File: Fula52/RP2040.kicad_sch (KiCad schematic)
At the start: 25 parts, among them SW1 BOOT, SW2 RESET, U3 W25Q128JVS, U4 RP2040, Y1 12MHz

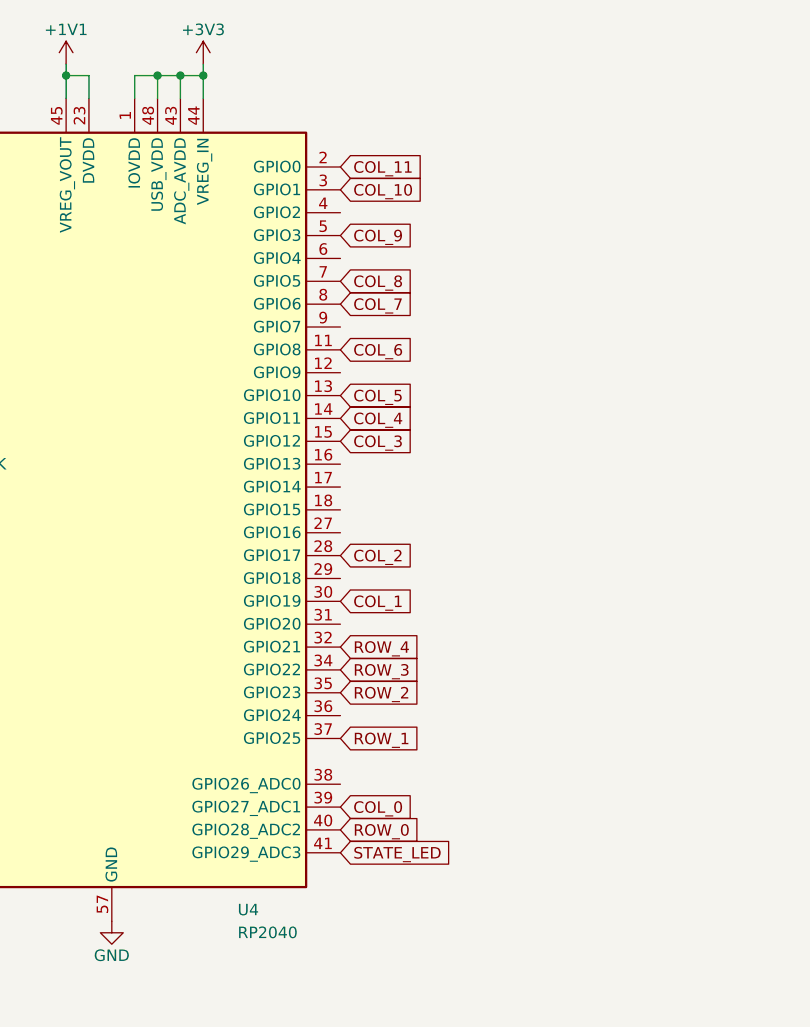
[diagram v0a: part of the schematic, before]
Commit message: full routed
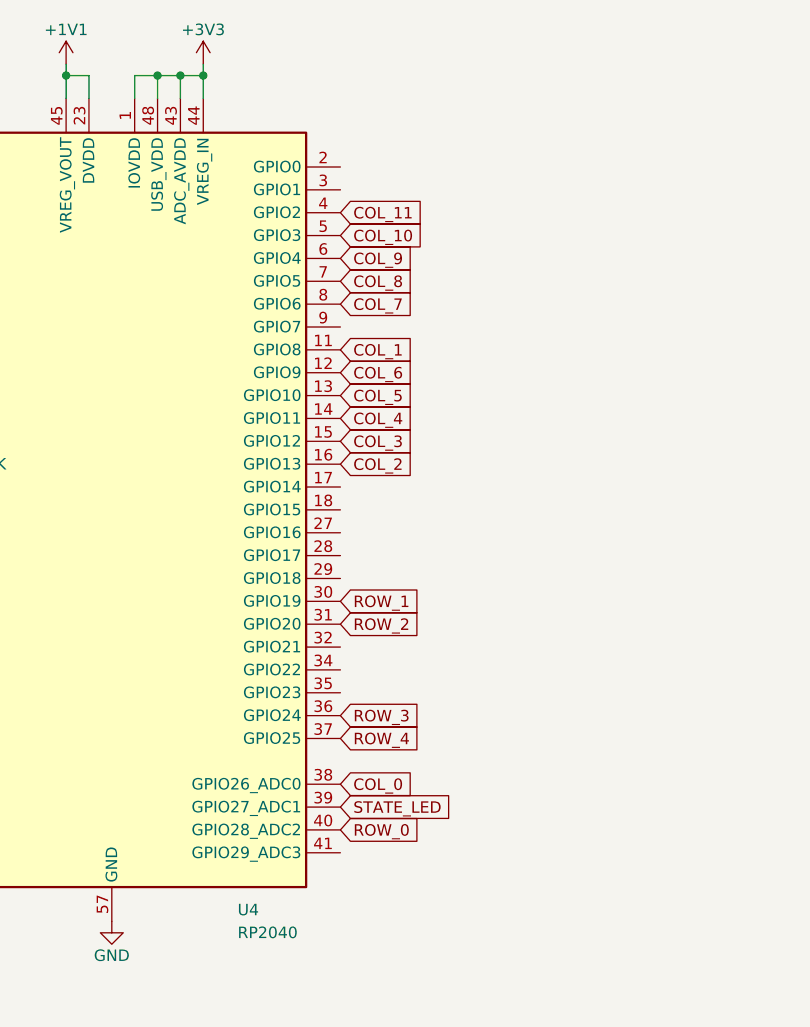
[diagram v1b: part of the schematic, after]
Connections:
- net COL_0: now also U4.38 (GPIO26_ADC0); no longer U4.39 (GPIO27_ADC1)
- net COL_1: now also U4.11 (GPIO8); no longer U4.30 (GPIO19)
- net COL_10: now also U4.5 (GPIO3); no longer U4.3 (GPIO1)
- net COL_11: now also U4.4 (GPIO2); no longer U4.2 (GPIO0)
- net COL_2: now also U4.16 (GPIO13); no longer U4.28 (GPIO17)
- net COL_6: now also U4.12 (GPIO9); no longer U4.11 (GPIO8)
- net COL_9: now also U4.6 (GPIO4); no longer U4.5 (GPIO3)
- net ROW_1: now also U4.30 (GPIO19); no longer U4.37 (GPIO25)
- net ROW_2: now also U4.31 (GPIO20); no longer U4.35 (GPIO23)
- net ROW_3: now also U4.36 (GPIO24); no longer U4.34 (GPIO22)
- net ROW_4: now also U4.37 (GPIO25); no longer U4.32 (GPIO21)
- net STATE_LED: now also U4.39 (GPIO27_ADC1); no longer U4.41 (GPIO29_ADC3)
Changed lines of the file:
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@@
     (effects (font (size 1.27 1.27)) (justify right bottom))
   )
-  (global_label "COL_2" (shape input) (at 116.84 83.82 0) (fields_autoplaced)
+  (global_label "COL_2" (shape input) (at 116.84 73.66 0) (fields_autoplaced)
     (effects (font (size 1.27 1.27)) (justify left))
-    (property "Intersheet References" "${INTERSHEET_REFS}" (id 0) (at 125.0588 83.7406 0)
+    (property "Intersheet References" "${INTERSHEET_REFS}" (id 0) (at 125.0588 73.5806 0)
       (effects (font (size 1.27 1.27)) (justify left) hide)
     )
   )
-  (global_label "ROW_1" (shape input) (at 116.84 104.14 0) (fields_autoplaced)
+  (global_label "ROW_1" (shape input) (at 116.84 88.9 0) (fields_autoplaced)
     (effects (font (size 1.27 1.27)) (justify left))
-    (property "Intersheet References" "${INTERSHEET_REFS}" (id 0) (at 125.4821 104.0606 0)
+    (property "Intersheet References" "${INTERSHEET_REFS}" (id 0) (at 125.4821 88.8206 0)
       (effects (font (size 1.27 1.27)) (justify left) hide)
     )
@@
     )
   )
-  (global_label "COL_10" (shape input) (at 116.84 43.18 0) (fields_autoplaced)
+  (global_label "COL_10" (shape input) (at 116.84 48.26 0) (fields_autoplaced)
     (effects (font (size 1.27 1.27)) (justify left))
-    (property "Intersheet References" "${INTERSHEET_REFS}" (id 0) (at 126.2683 43.1006 0)
+    (property "Intersheet References" "${INTERSHEET_REFS}" (id 0) (at 126.2683 48.1806 0)
       (effects (font (size 1.27 1.27)) (justify left) hide)
     )
@@
     )
   )
-  (global_label "COL_0" (shape input) (at 116.84 111.76 0) (fields_autoplaced)
+  (global_label "COL_0" (shape input) (at 116.84 109.22 0) (fields_autoplaced)
     (effects (font (size 1.27 1.27)) (justify left))
-    (property "Intersheet References" "${INTERSHEET_REFS}" (id 0) (at 125.0588 111.6806 0)
+    (property "Intersheet References" "${INTERSHEET_REFS}" (id 0) (at 125.0588 109.1406 0)
       (effects (font (size 1.27 1.27)) (justify left) hide)
     )
   )
-  (global_label "COL_9" (shape input) (at 116.84 48.26 0) (fields_autoplaced)
+  (global_label "COL_9" (shape input) (at 116.84 50.8 0) (fields_autoplaced)
     (effects (font (size 1.27 1.27)) (justify left))
-    (property "Intersheet References" "${INTERSHEET_REFS}" (id 0) (at 125.0588 48.1806 0)
+    (property "Intersheet References" "${INTERSHEET_REFS}" (id 0) (at 125.0588 50.7206 0)
       (effects (font (size 1.27 1.27)) (justify left) hide)
     )
   )
-  (global_label "ROW_4" (shape input) (at 116.84 93.98 0) (fields_autoplaced)
+  (global_label "ROW_4" (shape input) (at 116.84 104.14 0) (fields_autoplaced)
     (effects (font (size 1.27 1.27)) (justify left))
-    (property "Intersheet References" "${INTERSHEET_REFS}" (id 0) (at 125.4821 93.9006 0)
+    (property "Intersheet References" "${INTERSHEET_REFS}" (id 0) (at 125.4821 104.0606 0)
       (effects (font (size 1.27 1.27)) (justify left) hide)
     )
   )
-  (global_label "COL_11" (shape input) (at 116.84 40.64 0) (fields_autoplaced)
+  (global_label "COL_11" (shape input) (at 116.84 45.72 0) (fields_autoplaced)
     (effects (font (size 1.27 1.27)) (justify left))
-    (property "Intersheet References" "${INTERSHEET_REFS}" (id 0) (at 126.2683 40.5606 0)
+    (property "Intersheet References" "${INTERSHEET_REFS}" (id 0) (at 126.2683 45.6406 0)
       (effects (font (size 1.27 1.27)) (justify left) hide)
     )
@@
     )
   )
-  (global_label "COL_6" (shape input) (at 116.84 60.96 0) (fields_autoplaced)
+  (global_label "COL_6" (shape input) (at 116.84 63.5 0) (fields_autoplaced)
     (effects (font (size 1.27 1.27)) (justify left))
-    (property "Intersheet References" "${INTERSHEET_REFS}" (id 0) (at 125.0588 60.8806 0)
+    (property "Intersheet References" "${INTERSHEET_REFS}" (id 0) (at 125.0588 63.4206 0)
       (effects (font (size 1.27 1.27)) (justify left) hide)
     )
   )
-  (global_label "ROW_3" (shape input) (at 116.84 96.52 0) (fields_autoplaced)
+  (global_label "ROW_3" (shape input) (at 116.84 101.6 0) (fields_autoplaced)
     (effects (font (size 1.27 1.27)) (justify left))
-    (property "Intersheet References" "${INTERSHEET_REFS}" (id 0) (at 125.4821 96.4406 0)
+    (property "Intersheet References" "${INTERSHEET_REFS}" (id 0) (at 125.4821 101.5206 0)
       (effects (font (size 1.27 1.27)) (justify left) hide)
     )
@@
     )
   )
-  (global_label "ROW_2" (shape input) (at 116.84 99.06 0) (fields_autoplaced)
+  (global_label "ROW_2" (shape input) (at 116.84 91.44 0) (fields_autoplaced)
     (effects (font (size 1.27 1.27)) (justify left))
-    (property "Intersheet References" "${INTERSHEET_REFS}" (id 0) (at 125.4821 98.9806 0)
+    (property "Intersheet References" "${INTERSHEET_REFS}" (id 0) (at 125.4821 91.3606 0)
       (effects (font (size 1.27 1.27)) (justify left) hide)
     )
   )
-  (global_label "COL_1" (shape input) (at 116.84 88.9 0) (fields_autoplaced)
+  (global_label "COL_1" (shape input) (at 116.84 60.96 0) (fields_autoplaced)
     (effects (font (size 1.27 1.27)) (justify left))
-    (property "Intersheet References" "${INTERSHEET_REFS}" (id 0) (at 125.0588 88.8206 0)
+    (property "Intersheet References" "${INTERSHEET_REFS}" (id 0) (at 125.0588 60.8806 0)
       (effects (font (size 1.27 1.27)) (justify left) hide)
     )
   )
-  (global_label "STATE_LED" (shape input) (at 116.84 116.84 0) (fields_autoplaced)
+  (global_label "STATE_LED" (shape input) (at 116.84 111.76 0) (fields_autoplaced)
     (effects (font (size 1.27 1.27)) (justify left))
-    (property "Intersheet References" "${INTERSHEET_REFS}" (id 0) (at 129.0502 116.7606 0)
+    (property "Intersheet References" "${INTERSHEET_REFS}" (id 0) (at 129.0502 111.6806 0)
       (effects (font (size 1.27 1.27)) (justify left) hide)
     )
